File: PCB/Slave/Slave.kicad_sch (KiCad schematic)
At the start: 54 parts, among them J1 USB_C_Receptacle_USB2.0_16P, J2 Conn_01x05_Pin, J3 Conn_01x07_Socket, J4 Conn_01x04_Socket, J5 Conn_01x07_Socket, Q2 PNP, SW1 PTS810_SJM_250_SMTR_LFS, SW2 PTS810_SJM_250_SMTR_LFS, U1 ESP32-S3-MINI-1, U2 TCA9406DC, U3 BMP280, U4 P82B715D, U5 HX711, U6 SN65HVD230

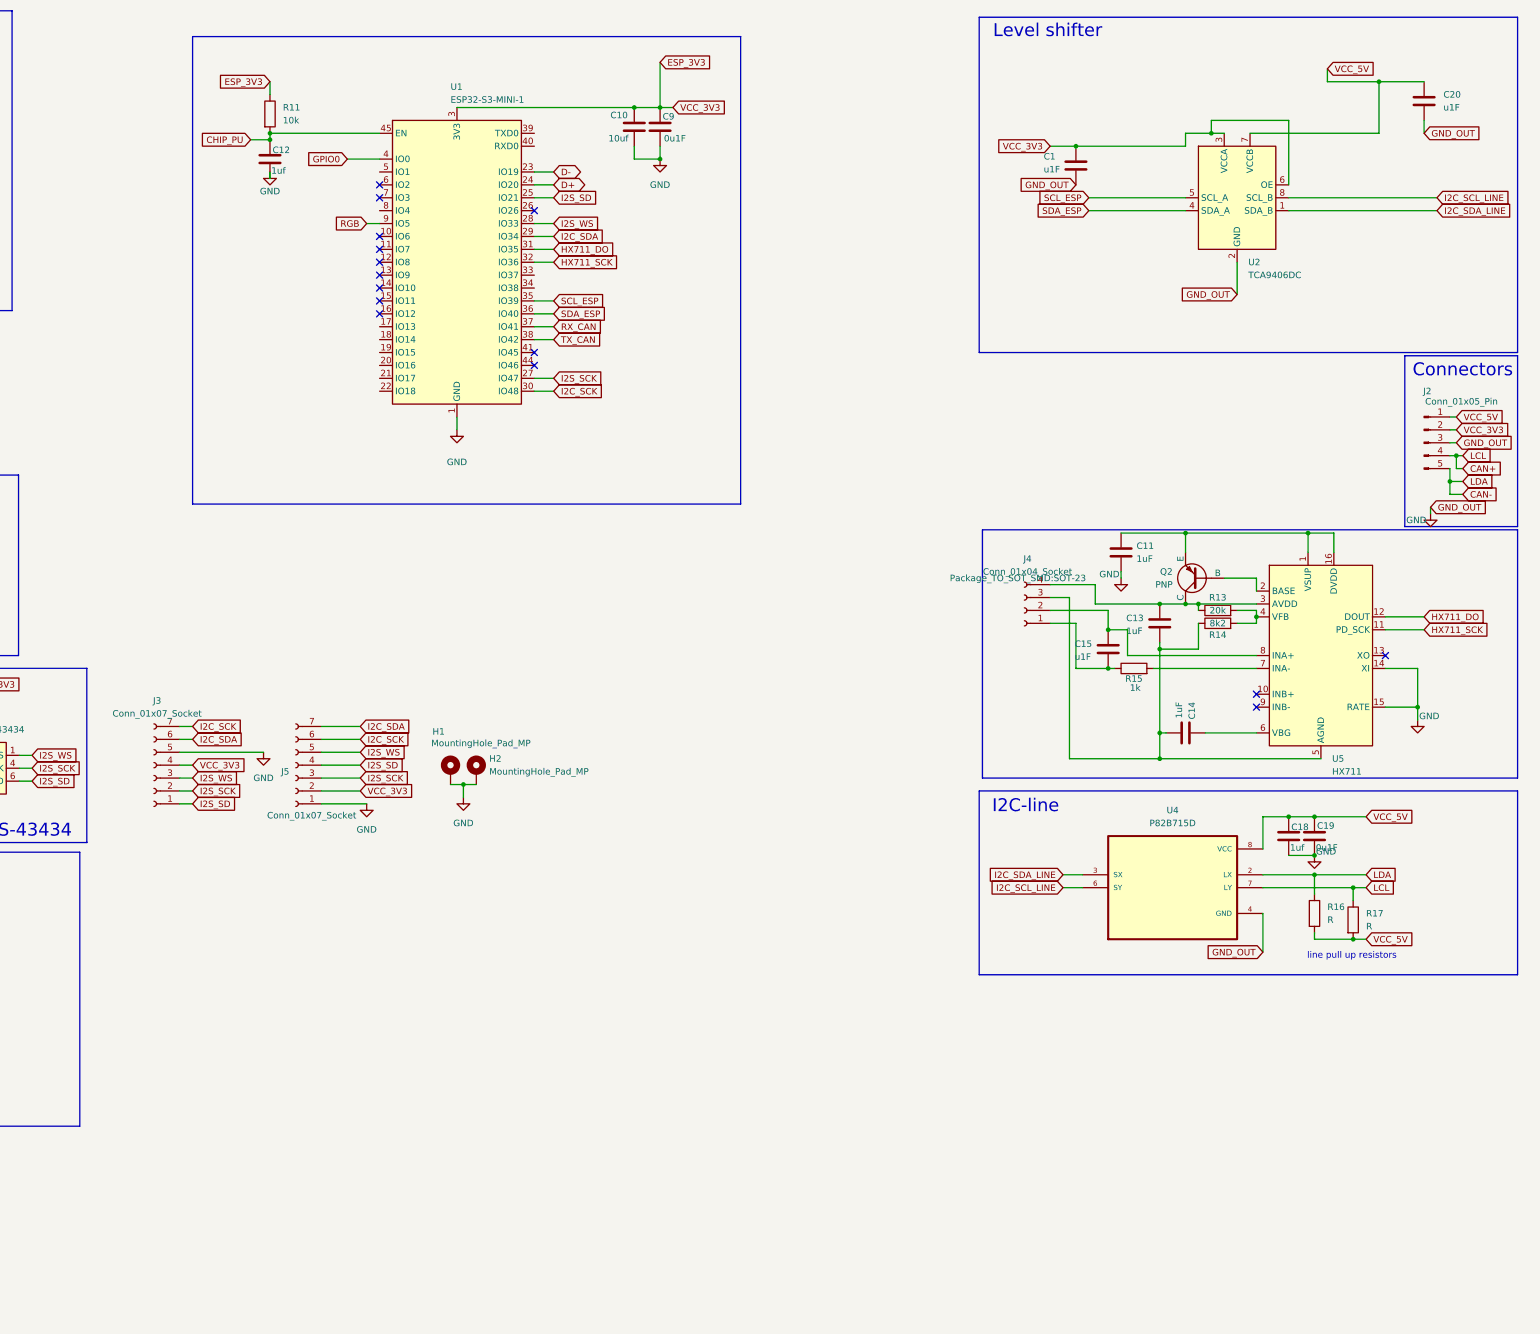
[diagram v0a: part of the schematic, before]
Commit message: PCB-Update
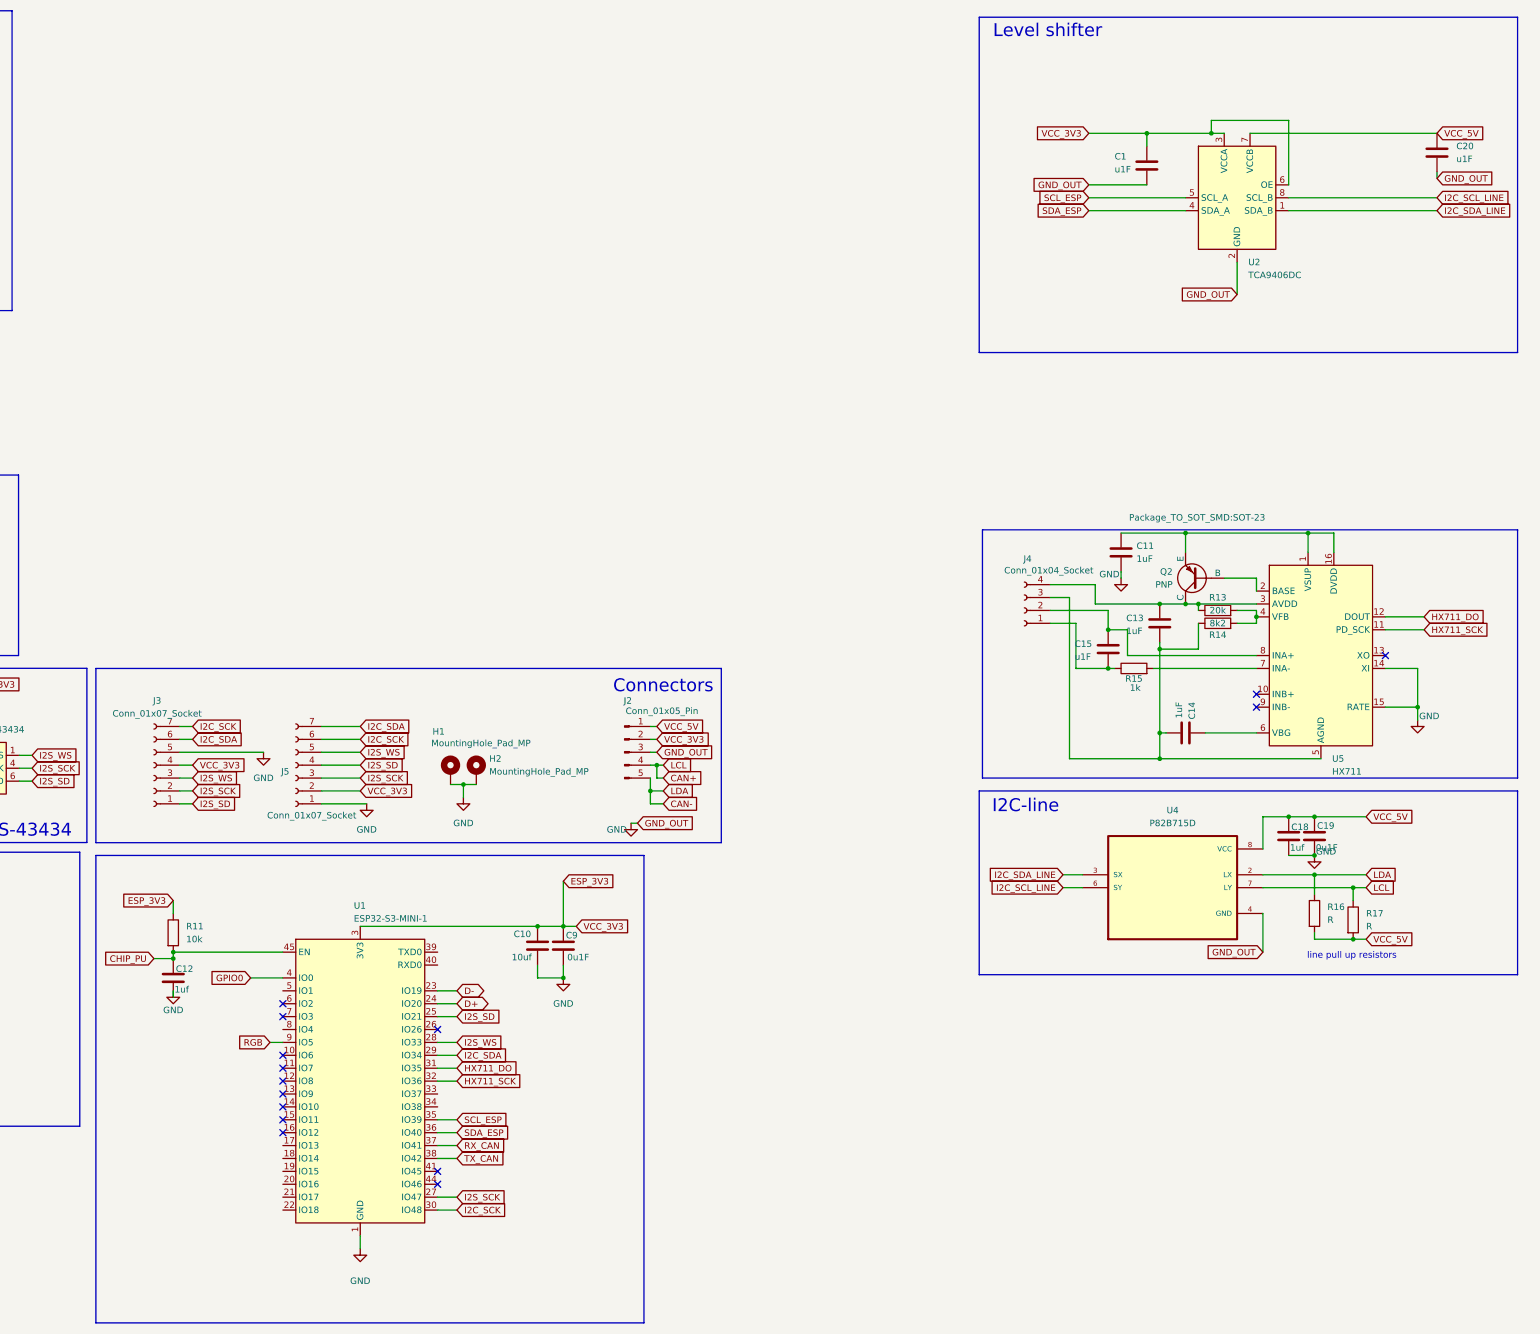
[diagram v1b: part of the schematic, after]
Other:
- moved on the sheet: C1, C10, C12, C20, C9, J2, R11, U1
